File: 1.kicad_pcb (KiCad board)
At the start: 2 copper layers, 77.5 x 40.6 mm, 24 parts, among them J1 Screw_Terminal_01x03, J2 Screw_Terminal_01x01, J3 Screw_Terminal_01x01, U1 LTC2990, U2 LTC2990, U3 LTC2990

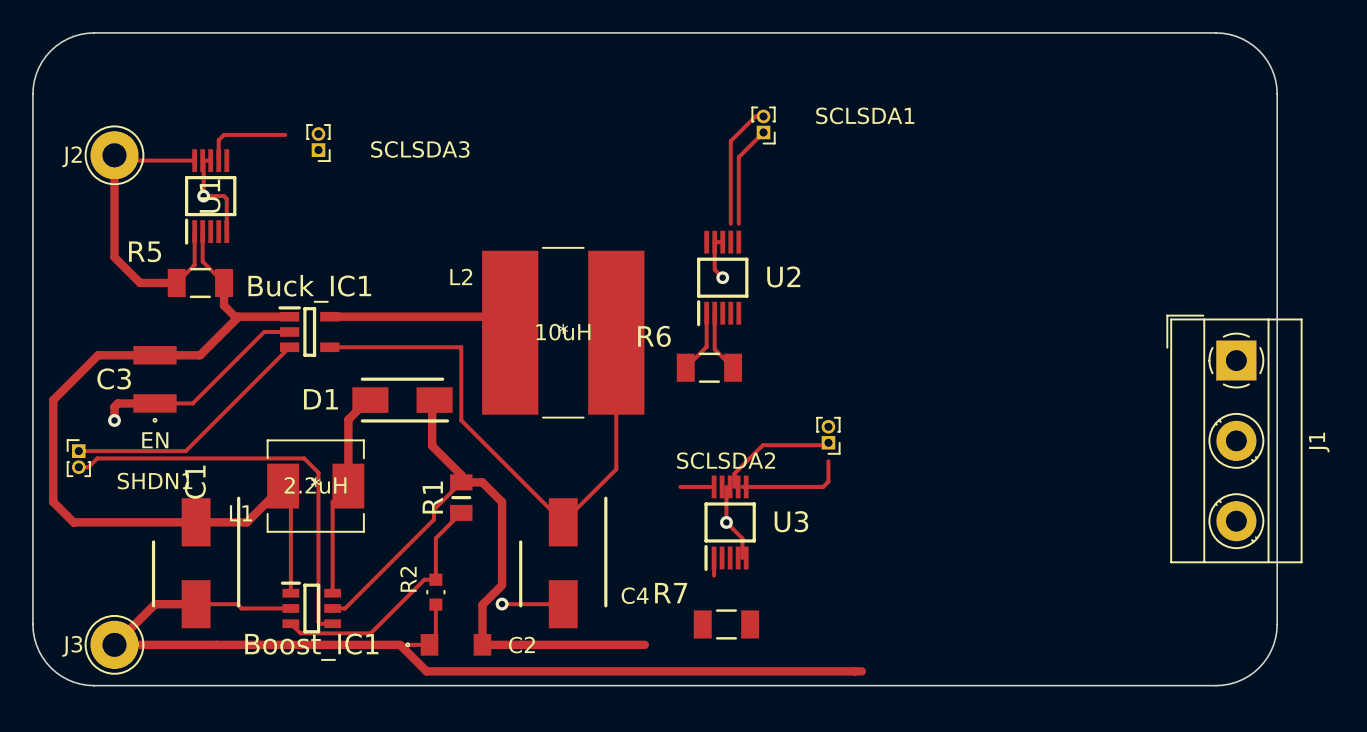
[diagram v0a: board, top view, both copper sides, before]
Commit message: v1
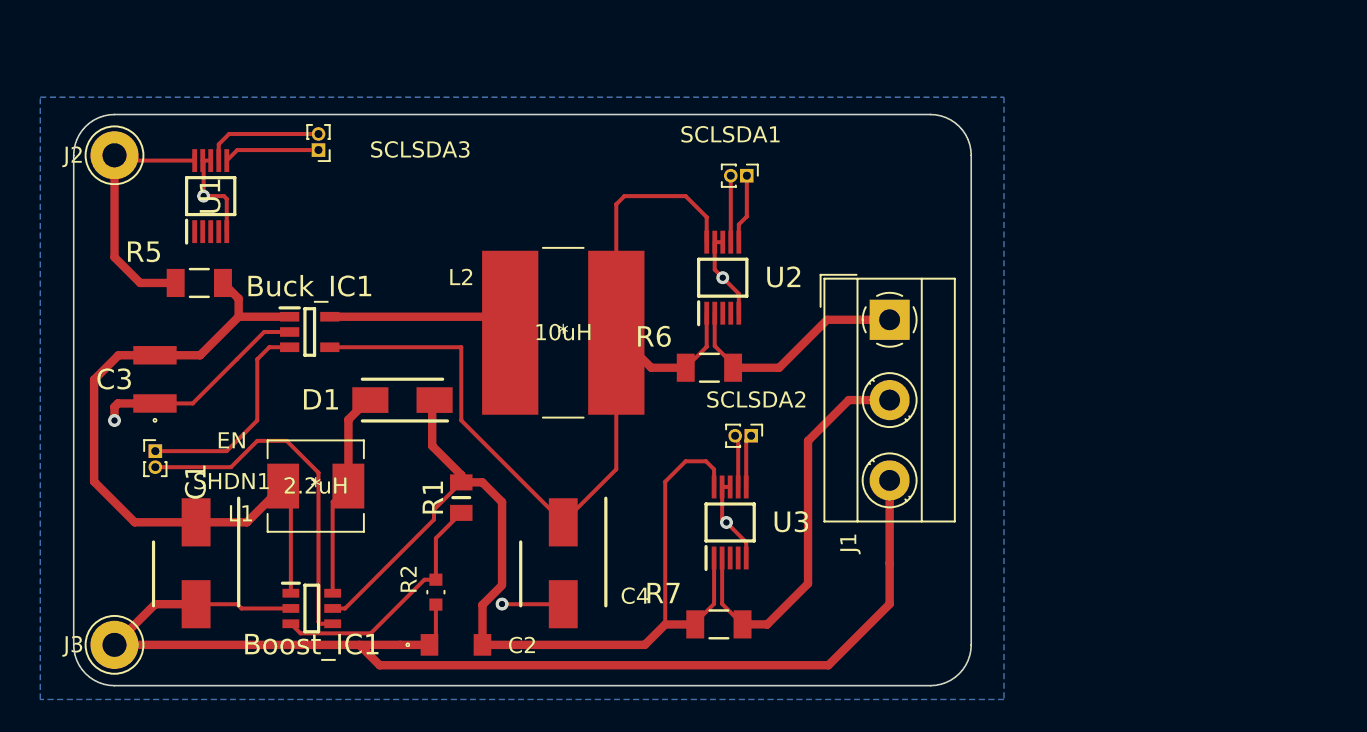
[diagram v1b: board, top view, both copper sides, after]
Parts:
- Boost_IC1: footprint Boost LTC3426:SOT95P280X90-6N -> libs:SOT95P280X90-6N
- Buck_IC1: footprint BUck TPS62203DBVT:SOT95P280X145-5N -> libs:SOT95P280X145-5N
- C1, C4: footprint capa 10uf:CAPAE530X610N -> libs:CAPAE530X610N
- C2: footprint cap 22uF low esr and esl:C3216_Commercial -> libs:C3216_Commercial
- C3: footprint cap 4.7uf:C1210 -> libs:C1210
- D1: footprint Schottky dd:DIOM5026X220N -> libs:DIOM5026X220N
- J1: footprint TerminalBlock_MetzConnect:TerminalBlock_MetzConnect_Type055_RT01503HDWU_1x03_P5.00mm_Horizontal -> libs:TerminalBlock_MetzConnect_Type055_RT01503HDWU_1x03_P5.00mm_Horizontal
- J2, J3: footprint Connector_Pin:Pin_D1.3mm_L11.0mm_LooseFit -> libs:Pin_D1.3mm_L11.0mm_LooseFit
- L1: footprint indc 2.2uH:IHLP2020CZER2R2M8A -> libs:IHLP2020CZER2R2M8A
- L2: footprint indc 10uH crct:SRN1060-100M -> libs:SRN1060-100M
- R1: footprint rst 95.3k:RESC2012X60N -> libs:RESC2012X60N
- R2: footprint rst 30.9k:RC0603FR-0730K9L -> libs:RC0603FR-0730K9L
- R5, R6, R7: footprint 50m RST:RESC3216X88N -> libs:RESC3216X88N
- SCLSDA1, SCLSDA2, SCLSDA3, SHDN1: footprint Connector_PinHeader_1.00mm:PinHeader_1x02_P1.00mm_Vertical -> libs:PinHeader_1x02_P1.00mm_Vertical
- U1, U2, U3: footprint MON & PROTECC:SOP50P490X110-10N -> libs:SOP50P490X110-10N
- moved J1 21.7 mm to (182.9, 81.4)
- moved SCLSDA2 4.83 mm to (174.3, 88.6), turned to -90 degrees
- moved SHDN1 4.76 mm to (137.2, 89.5)
- moved SCLSDA1 2.88 mm to (174.0, 72.4), turned to -90 degrees
- moved R7 0.47 mm to (172.2, 100.3)
- moved R5 0.07 mm to (139.9, 79.1)
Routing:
- net Net-(J1-Pad2): track 0.00 -> 24.8 mm
- net Earth: track 90.6 -> 112.1 mm
- net Net-(Buck_IC1-Pad4): track 38.8 -> 60.0 mm
- net Net-(Boost_IC1-Pad5): track 43.2 -> 62.3 mm
- net Net-(SCLSDA2-Pad1): track 19.0 -> 3.31 mm
- net Net-(J1-Pad1): track 3.87 -> 14.9 mm
- net Net-(Boost_IC1-Pad1): track 52.2 -> 43.4 mm
- net Net-(SCLSDA3-Pad1): track 0.00 -> 5.98 mm
- net Net-(Boost_IC1-Pad4): track 25.7 -> 21.9 mm
- net Net-(J2-Pad1): track 20.1 -> 16.4 mm
- net Net-(SCLSDA1-Pad2): track 7.82 -> 4.14 mm
- net Net-(SCLSDA2-Pad2): track 0.00 -> 3.26 mm
- net Net-(Buck_IC1-Pad3): track 15.8 -> 13.3 mm
- net Net-(SCLSDA1-Pad1): track 6.32 -> 4.35 mm
- net Net-(SCLSDA3-Pad2): track 5.54 -> 7.49 mm
- added copper zone on B.Cu, net Earth
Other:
- board size 77.5 x 40.6 mm -> 55.9 x 35.6 mm
